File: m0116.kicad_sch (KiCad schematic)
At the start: 262 parts, among them J1 Conn_01x04, J2 Conn_01x04_MountingPin, J3 Conn_01x04_MountingPin, J4 Conn_01x04, J7 Conn_01x05, Q1 Q_PMOS_GSD AO3401A, Q2 Q_NMOS_GSD 2N7002, Q3 Q_NMOS_GSD 2N7002, Q4 2N3904, SW1 SW_Push, U1 XC6206P332MR, U2 74AHCT1G125, U3 STM32F411RETx, U4 24LC64, U5 USBLC6-2SC6, Y1 8MHz

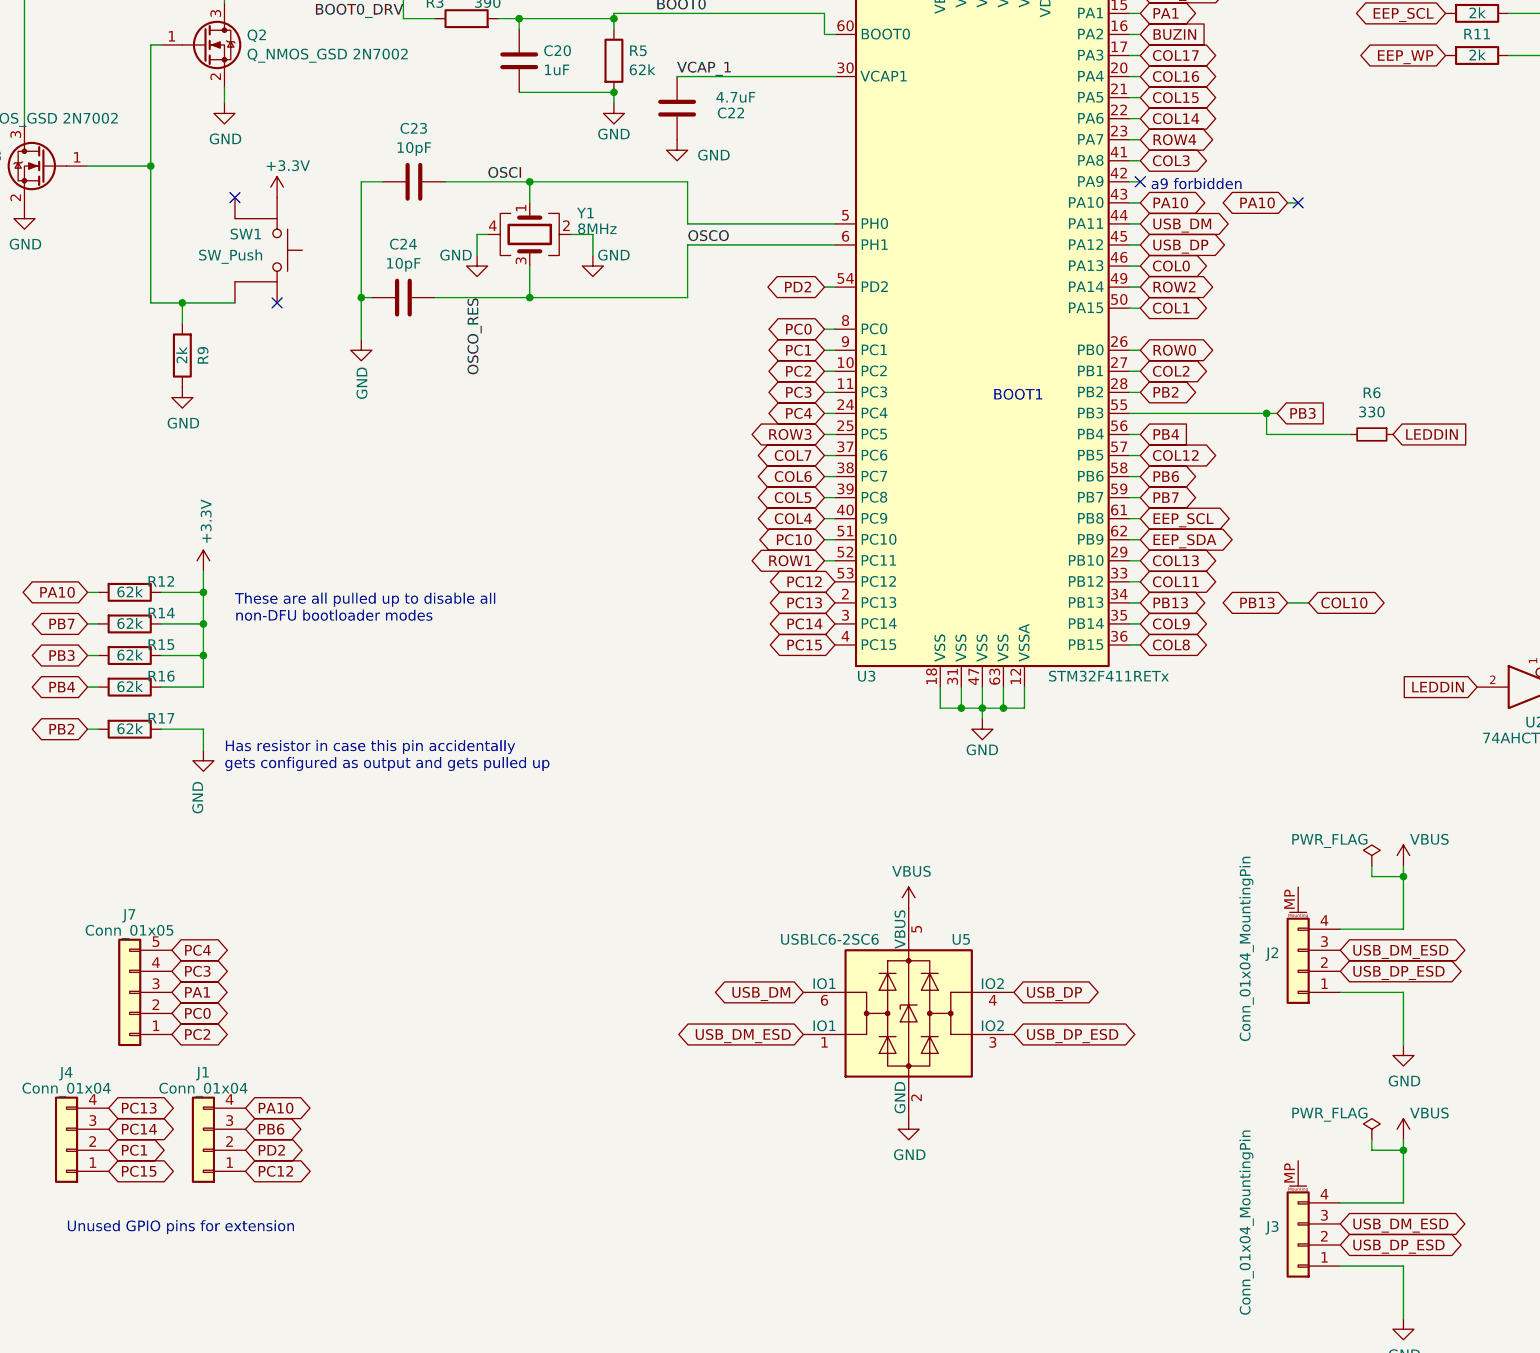
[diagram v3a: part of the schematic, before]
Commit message: updates
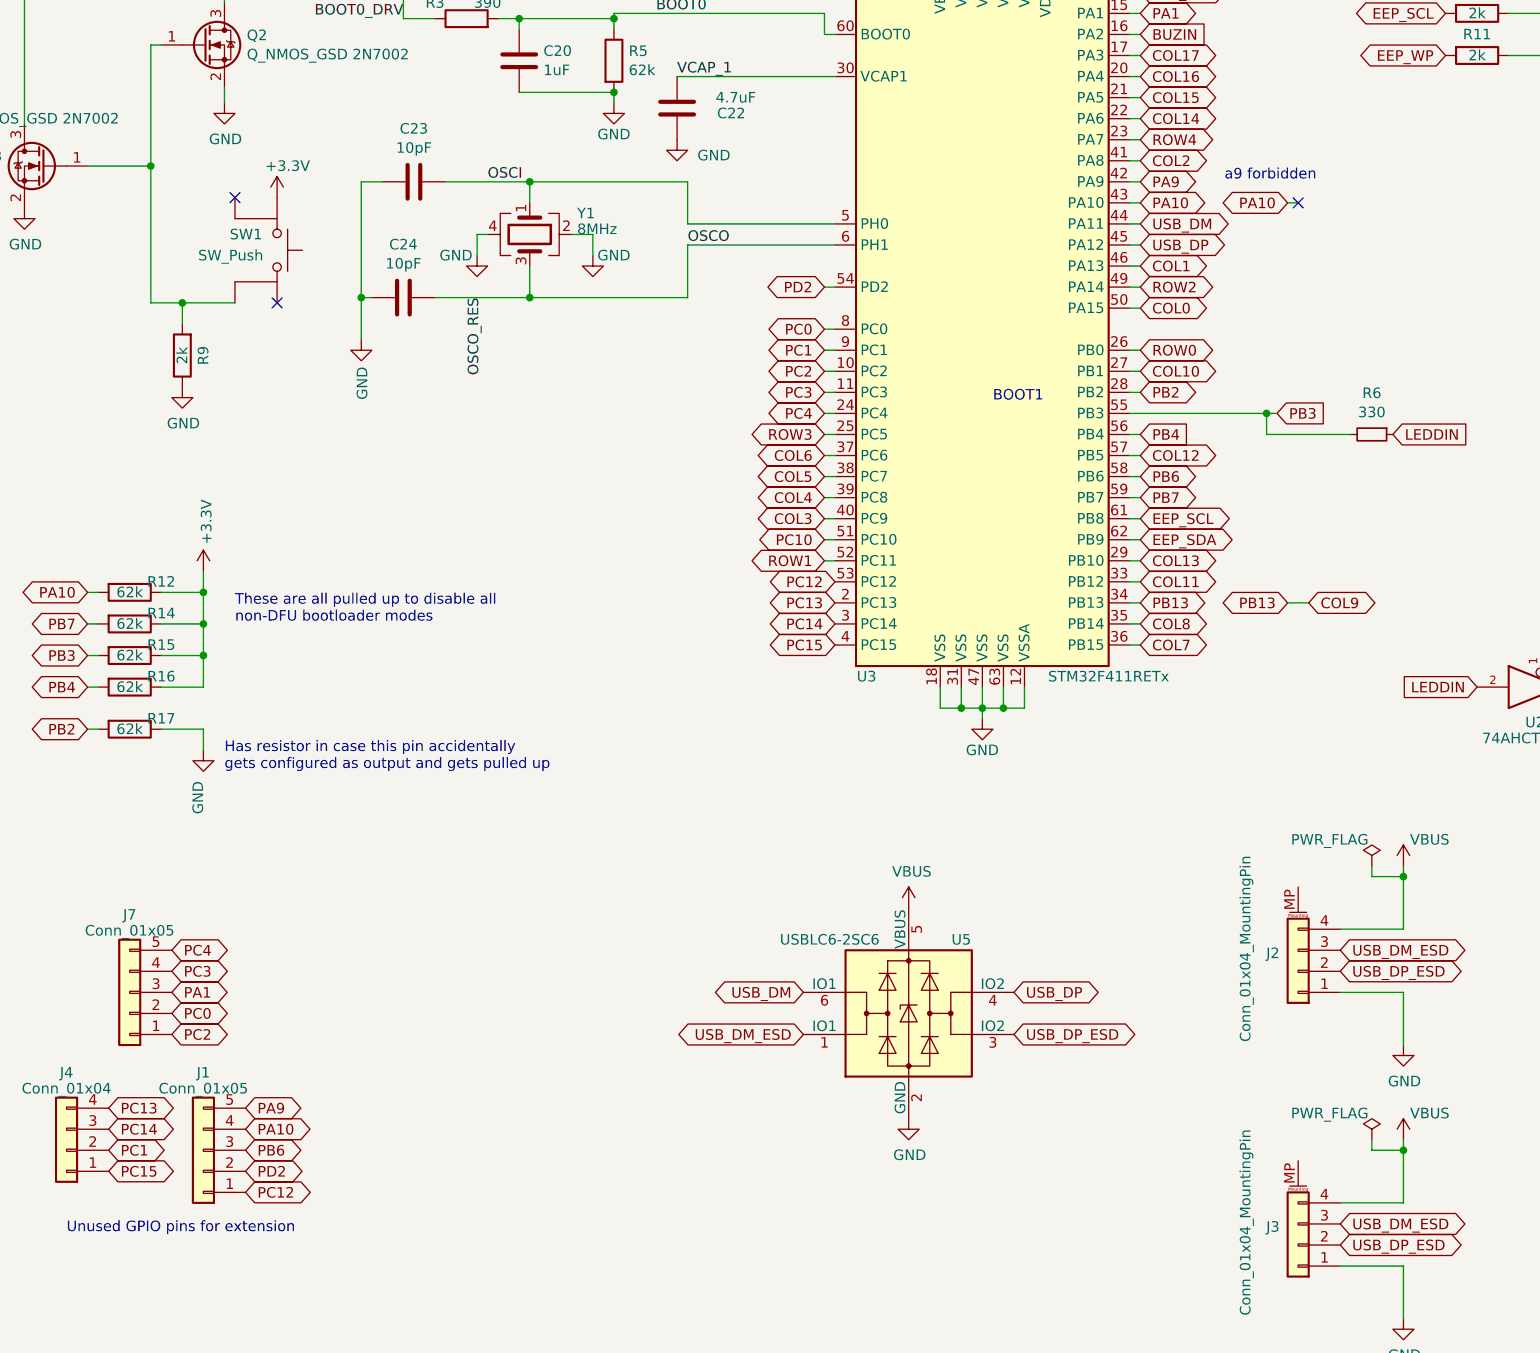
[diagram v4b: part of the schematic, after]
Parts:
- J1: value Conn_01x04 -> Conn_01x05; footprint Connector_PinHeader_1.27mm:PinHeader_1x04_P1.27mm_Vertical -> Connector_PinHeader_1.27mm:PinHeader_1x05_P1.27mm_Vertical; symbol Connector_Generic:Conn_01x04 -> Connector_Generic:Conn_01x05
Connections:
- net COL0: now also U3.50 (PA15); no longer U3.46 (PA13)
- net COL1: now also U3.46 (PA13); no longer U3.50 (PA15)
- net COL10: now also U3.27 (PB1); no longer U3.34 (PB13)
- net COL2: now also U3.41 (PA8); no longer U3.27 (PB1)
- net COL3: now also U3.40 (PC9); no longer U3.41 (PA8)
- net COL4: now also U3.39 (PC8); no longer U3.40 (PC9)
- net COL5: now also U3.38 (PC7); no longer U3.39 (PC8)
- net COL6: now also U3.37 (PC6); no longer U3.38 (PC7)
- net COL7: now also U3.36 (PB15); no longer U3.37 (PC6)
- net COL8: now also U3.35 (PB14); no longer U3.36 (PB15)
- net COL9: now also U3.34 (PB13); no longer U3.35 (PB14)
- net PA9: now reaches U3.42 (PA9)
- net PA9: now also J1.5 (Pin_5)
- no-connect marks 4 -> 3
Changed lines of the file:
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@@
   )
   (no_connect (at 58.42 118.745))
-  (no_connect (at 162.56 104.14))
   (no_connect (at 181.61 106.68))
   (no_connect (at 53.34 106.045))
@@
     (effects (font (size 1.0922 1.0922)) (justify left bottom))
   )
-  (text "a9 forbidden\n" (at 163.83 105.41 0)
+  (text "a9 forbidden\n" (at 172.72 104.14 0)
     (effects (font (size 1.27 1.27)) (justify left bottom))
   )
@@
     )
   )
-  (global_label "COL10" (shape bidirectional) (at 182.88 154.94 0)
+  (global_label "COL10" (shape bidirectional) (at 162.56 127 0)
     (effects (font (size 1.27 1.27)) (justify left))
-    (property "Intersheetrefs" "${INTERSHEET_REFS}" (at 182.88 154.94 0)
+    (property "Intersheetrefs" "${INTERSHEET_REFS}" (at 162.56 127 0)
       (effects (font (size 1.27 1.27)) hide)
     )
@@
     )
   )
-  (global_label "COL3" (shape bidirectional) (at 162.56 101.6 0)
-    (effects (font (size 1.27 1.27)) (justify left))
-    (property "Intersheetrefs" "${INTERSHEET_REFS}" (at 162.56 101.6 0)
+  (global_label "COL3" (shape bidirectional) (at 124.46 144.78 180)
+    (effects (font (size 1.27 1.27)) (justify right))
+    (property "Intersheetrefs" "${INTERSHEET_REFS}" (at 124.46 144.78 0)
       (effects (font (size 1.27 1.27)) hide)
     )
@@
     )
   )
-  (global_label "COL5" (shape bidirectional) (at 124.46 142.24 180)
+  (global_label "COL5" (shape bidirectional) (at 124.46 139.7 180)
     (effects (font (size 1.27 1.27)) (justify right))
-    (property "Intersheetrefs" "${INTERSHEET_REFS}" (at 124.46 142.24 0)
+    (property "Intersheetrefs" "${INTERSHEET_REFS}" (at 124.46 139.7 0)
       (effects (font (size 1.27 1.27)) hide)
     )
@@
     )
   )
-  (global_label "COL1" (shape bidirectional) (at 162.56 119.38 0)
+  (global_label "COL1" (shape bidirectional) (at 162.56 114.3 0)
     (effects (font (size 1.27 1.27)) (justify left))
-    (property "Intersheetrefs" "${INTERSHEET_REFS}" (at 162.56 119.38 0)
+    (property "Intersheetrefs" "${INTERSHEET_REFS}" (at 162.56 114.3 0)
       (effects (font (size 1.27 1.27)) hide)
     )
@@
     )
   )
-  (global_label "COL9" (shape bidirectional) (at 162.56 157.48 0)
+  (global_label "COL9" (shape bidirectional) (at 182.88 154.94 0)
     (effects (font (size 1.27 1.27)) (justify left))
-    (property "Intersheetrefs" "${INTERSHEET_REFS}" (at 162.56 157.48 0)
+    (property "Intersheetrefs" "${INTERSHEET_REFS}" (at 182.88 154.94 0)
       (effects (font (size 1.27 1.27)) hide)
     )
@@
     )
   )
-  (global_label "PB6" (shape bidirectional) (at 54.61 218.44 0)
+  (global_label "PB6" (shape bidirectional) (at 54.61 220.98 0)
     (effects (font (size 1.27 1.27)) (justify left))
-    (property "Intersheetrefs" "${INTERSHEET_REFS}" (at 54.61 218.44 0)
+    (property "Intersheetrefs" "${INTERSHEET_REFS}" (at 54.61 220.98 0)
       (effects (font (size 1.27 1.27)) hide)
     )
@@
     )
   )
-  (global_label "COL4" (shape bidirectional) (at 124.46 144.78 180)
+  (global_label "COL4" (shape bidirectional) (at 124.46 142.24 180)
     (effects (font (size 1.27 1.27)) (justify right))
-    (property "Intersheetrefs" "${INTERSHEET_REFS}" (at 124.46 144.78 0)
+    (property "Intersheetrefs" "${INTERSHEET_REFS}" (at 124.46 142.24 0)
       (effects (font (size 1.27 1.27)) hide)
     )
@@
     )
   )
-  (global_label "COL7" (shape bidirectional) (at 124.46 137.16 180)
-    (effects (font (size 1.27 1.27)) (justify right))
-    (property "Intersheetrefs" "${INTERSHEET_REFS}" (at 124.46 137.16 0)
+  (global_label "COL7" (shape bidirectional) (at 162.56 160.02 0)
+    (effects (font (size 1.27 1.27)) (justify left))
+    (property "Intersheetrefs" "${INTERSHEET_REFS}" (at 162.56 160.02 0)
       (effects (font (size 1.27 1.27)) hide)
     )
@@
     )
   )
-  (global_label "COL8" (shape bidirectional) (at 162.56 160.02 0)
+  (global_label "COL8" (shape bidirectional) (at 162.56 157.48 0)
     (effects (font (size 1.27 1.27)) (justify left))
-    (property "Intersheetrefs" "${INTERSHEET_REFS}" (at 162.56 160.02 0)
+    (property "Intersheetrefs" "${INTERSHEET_REFS}" (at 162.56 157.48 0)
       (effects (font (size 1.27 1.27)) hide)
     )
@@
     )
   )
-  (global_label "PD2" (shape bidirectional) (at 54.61 220.98 0)
+  (global_label "PD2" (shape bidirectional) (at 54.61 223.52 0)
     (effects (font (size 1.27 1.27)) (justify left))
-    (property "Intersheetrefs" "${INTERSHEET_REFS}" (at 54.61 220.98 0)
+    (property "Intersheetrefs" "${INTERSHEET_REFS}" (at 54.61 223.52 0)
       (effects (font (size 1.27 1.27)) hide)
     )
@@
     )
   )
-  (global_label "COL6" (shape bidirectional) (at 124.46 139.7 180)
+  (global_label "COL6" (shape bidirectional) (at 124.46 137.16 180)
     (effects (font (size 1.27 1.27)) (justify right))
-    (property "Intersheetrefs" "${INTERSHEET_REFS}" (at 124.46 139.7 0)
+    (property "Intersheetrefs" "${INTERSHEET_REFS}" (at 124.46 137.16 0)
       (effects (font (size 1.27 1.27)) hide)
     )
@@
     )
   )
-  (global_label "PA10" (shape bidirectional) (at 54.61 215.9 0)
+  (global_label "PA10" (shape bidirectional) (at 54.61 218.44 0)
     (effects (font (size 1.27 1.27)) (justify left))
-    (property "Intersheetrefs" "${INTERSHEET_REFS}" (at 54.61 215.9 0)
+    (property "Intersheetrefs" "${INTERSHEET_REFS}" (at 54.61 218.44 0)
       (effects (font (size 1.27 1.27)) hide)
     )
@@
     )
   )
-  (global_label "PC12" (shape bidirectional) (at 54.61 223.52 0)
+  (global_label "PC12" (shape bidirectional) (at 54.61 226.06 0)
     (effects (font (size 1.27 1.27)) (justify left))
-    (property "Intersheetrefs" "${INTERSHEET_REFS}" (at 54.61 223.52 0)
+    (property "Intersheetrefs" "${INTERSHEET_REFS}" (at 54.61 226.06 0)
       (effects (font (size 1.27 1.27)) hide)
     )
@@
     )
   )
-  (global_label "COL2" (shape bidirectional) (at 162.56 127 0)
+  (global_label "COL2" (shape bidirectional) (at 162.56 101.6 0)
     (effects (font (size 1.27 1.27)) (justify left))
-    (property "Intersheetrefs" "${INTERSHEET_REFS}" (at 162.56 127 0)
+    (property "Intersheetrefs" "${INTERSHEET_REFS}" (at 162.56 101.6 0)
       (effects (font (size 1.27 1.27)) hide)
     )
@@
     )
   )
+  (global_label "PA9" (shape bidirectional) (at 54.61 215.9 0)
+    (effects (font (size 1.27 1.27)) (justify left))
+    (property "Intersheetrefs" "${INTERSHEET_REFS}" (at 54.61 215.9 0)
+      (effects (font (size 1.27 1.27)) hide)
+    )
+  )
   (global_label "ROW0" (shape bidirectional) (at 162.56 124.46 0)
     (effects (font (size 1.27 1.27)) (justify left))
@@
     )
   )
-  (global_label "COL0" (shape bidirectional) (at 162.56 114.3 0)
+  (global_label "COL0" (shape bidirectional) (at 162.56 119.38 0)
     (effects (font (size 1.27 1.27)) (justify left))
-    (property "Intersheetrefs" "${INTERSHEET_REFS}" (at 162.56 114.3 0)
+    (property "Intersheetrefs" "${INTERSHEET_REFS}" (at 162.56 119.38 0)
       (effects (font (size 1.27 1.27)) hide)
     )
@@
     )
   )
+  (global_label "PA9" (shape bidirectional) (at 162.56 104.14 0)
+    (effects (font (size 1.27 1.27)) (justify left))
+    (property "Intersheetrefs" "${INTERSHEET_REFS}" (at 162.56 104.14 0)
+      (effects (font (size 1.27 1.27)) hide)
+    )
+  )
   (symbol (lib_id "ws2812b:WS2812B") (at 274.32 135.89 0) (unit 1)
     (in_bom yes) (on_board yes) (dnp no)
@@
     )
   )
-  (symbol (lib_id "Connector_Generic:Conn_01x04") (at 49.53 220.98 180) (unit 1)
+  (symbol (lib_id "Connector_Generic:Conn_01x05") (at 49.53 220.98 180) (unit 1)
     (in_bom yes) (on_board yes) (dnp no) (fields_autoplaced)
     (property "Reference" "J1" (at 49.53 211.6201 0)
       (effects (font (size 1.27 1.27)))
     )
-    (property "Value" "Conn_01x04" (at 49.53 213.5411 0)
+    (property "Value" "Conn_01x05" (at 49.53 213.5411 0)
       (effects (font (size 1.27 1.27)))
     )
-    (property "Footprint" "Connector_PinHeader_1.27mm:PinHeader_1x04_P1.27mm_Vertical" (at 49.53 220.98 0)
+    (property "Footprint" "Connector_PinHeader_1.27mm:PinHeader_1x05_P1.27mm_Vertical" (at 49.53 220.98 0)
       (effects (font (size 1.27 1.27)) hide)
     )
@@
     (pin "3")
     (pin "4")
+    (pin "5")
     (instances
       (project "m0116"

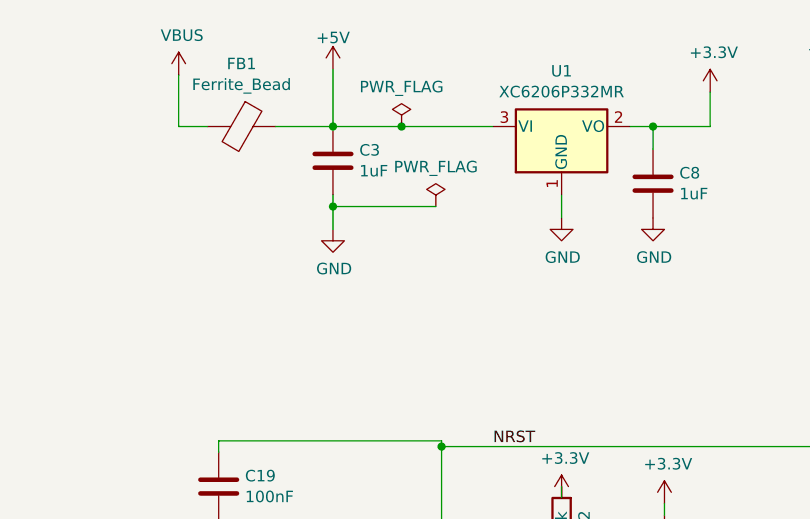
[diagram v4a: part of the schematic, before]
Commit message: fix
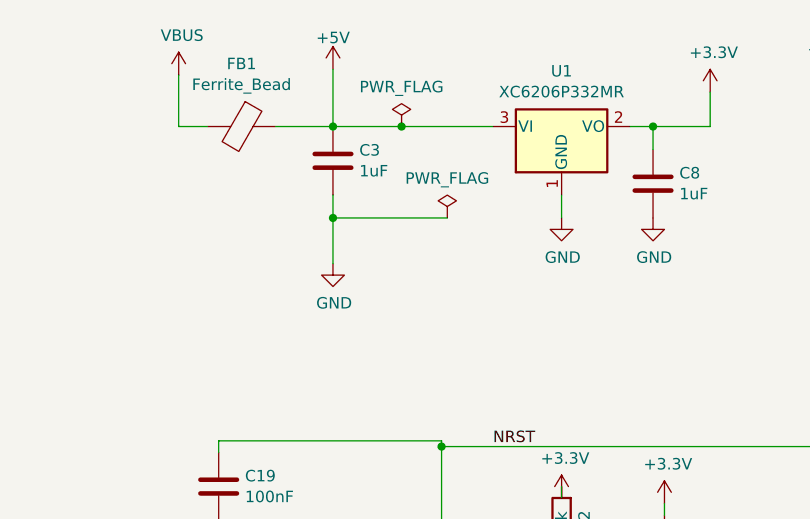
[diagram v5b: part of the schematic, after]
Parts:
- SW1: footprint random-keyboard-parts:SKQG-1155865 -> controller:switch_K2-1187SQ-A4SW-06
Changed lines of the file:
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@@
   (junction (at 160.02 314.96) (diameter 0) (color 0 0 0 0)
   )
-  (junction (at 36.83 35.56) (diameter 0) (color 0 0 0 0)
-  )
   (junction (at 143.51 361.95) (diameter 0) (color 0 0 0 0)
   )
@@
   (junction (at 167.64 323.85) (diameter 0) (color 0 0 0 0)
   )
+  (junction (at 36.83 36.83) (diameter 0) (color 0 0 0 0)
+  )
   (junction (at 86.36 386.08) (diameter 0) (color 0 0 0 0)
   )
@@
     (stroke (width 0) (type default))
   )
+  (wire (pts (xy 36.83 34.29) (xy 36.83 36.83))
+    (stroke (width 0) (type default))
+  )
   (wire (pts (xy 40.64 266.7) (xy 40.64 285.75))
     (stroke (width 0) (type solid))
@@
     (stroke (width 0) (type default))
   )
-  (wire (pts (xy 36.83 35.56) (xy 36.83 34.29))
-    (stroke (width 0) (type default))
-  )
   (wire (pts (xy 78.74 104.14) (xy 88.9 104.14))
     (stroke (width 0) (type default))
@@
     (stroke (width 0) (type solid))
   )
-  (wire (pts (xy 48.26 35.56) (xy 36.83 35.56))
+  (wire (pts (xy 49.53 36.83) (xy 36.83 36.83))
     (stroke (width 0) (type default))
   )
@@
     (stroke (width 0) (type default))
   )
-  (wire (pts (xy 36.83 38.1) (xy 36.83 35.56))
+  (wire (pts (xy 36.83 41.91) (xy 36.83 36.83))
     (stroke (width 0) (type default))
   )
@@
     )
   )
-  (symbol (lib_id "controller-rescue:GND-power") (at 36.83 38.1 0) (unit 1)
+  (symbol (lib_id "controller-rescue:GND-power") (at 36.83 41.91 0) (unit 1)
     (in_bom yes) (on_board yes) (dnp no)
-    (property "Reference" "#PWR023" (at 36.83 44.45 0)
+    (property "Reference" "#PWR023" (at 36.83 48.26 0)
       (effects (font (size 1.27 1.27)) hide)
     )
-    (property "Value" "GND" (at 36.957 42.4942 0)
+    (property "Value" "GND" (at 36.957 46.3042 0)
       (effects (font (size 1.27 1.27)))
     )
-    (property "Footprint" "" (at 36.83 38.1 0)
+    (property "Footprint" "" (at 36.83 41.91 0)
       (effects (font (size 1.27 1.27)) hide)
     )
-    (property "Datasheet" "" (at 36.83 38.1 0)
+    (property "Datasheet" "" (at 36.83 41.91 0)
       (effects (font (size 1.27 1.27)) hide)
     )
@@
       (effects (font (size 1.27 1.27)) (justify left))
     )
-    (property "Footprint" "random-keyboard-parts:SKQG-1155865" (at 63.5 112.395 0)
+    (property "Footprint" "controller:switch_K2-1187SQ-A4SW-06" (at 63.5 112.395 0)
       (effects (font (size 1.27 1.27)) hide)
     )
@@
     )
   )
-  (symbol (lib_id "controller-rescue:PWR_FLAG-power") (at 48.26 35.56 0) (unit 1)
+  (symbol (lib_id "controller-rescue:PWR_FLAG-power") (at 49.53 36.83 0) (unit 1)
     (in_bom yes) (on_board yes) (dnp no)
-    (property "Reference" "#FLG0103" (at 48.26 33.655 0)
+    (property "Reference" "#FLG0103" (at 49.53 34.925 0)
       (effects (font (size 1.27 1.27)) hide)
     )
-    (property "Value" "PWR_FLAG" (at 48.26 31.1658 0)
+    (property "Value" "PWR_FLAG" (at 49.53 32.4358 0)
       (effects (font (size 1.27 1.27)))
     )
-    (property "Footprint" "" (at 48.26 35.56 0)
+    (property "Footprint" "" (at 49.53 36.83 0)
       (effects (font (size 1.27 1.27)) hide)
     )
-    (property "Datasheet" "~" (at 48.26 35.56 0)
+    (property "Datasheet" "~" (at 49.53 36.83 0)
       (effects (font (size 1.27 1.27)) hide)
     )
